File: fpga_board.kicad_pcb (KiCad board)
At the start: 8 copper layers, 50 x 50 mm, 157 parts, among them Q1 2N7002PW, Q2 2N7002PW, Q3 2N7002PW, Q4 2N7002PW, Q5 2N7002PW, Q6 2N7002PW, SW1 1TS028A-1300-0600-CT, U1 LFE5U-45F-7BG256I, U10 TLV62569DRL, U2 CYUSB3014-BZXC, U3 TLV62569DRL, U5 K4B4G1646E-BCMA, U6 K4B4G1646E-BCMA, U7 TLV62569DRL, U8 TLV62569DRL, U9 TLV62569DRL, X1 XO32, Y1 Crystal_GND24

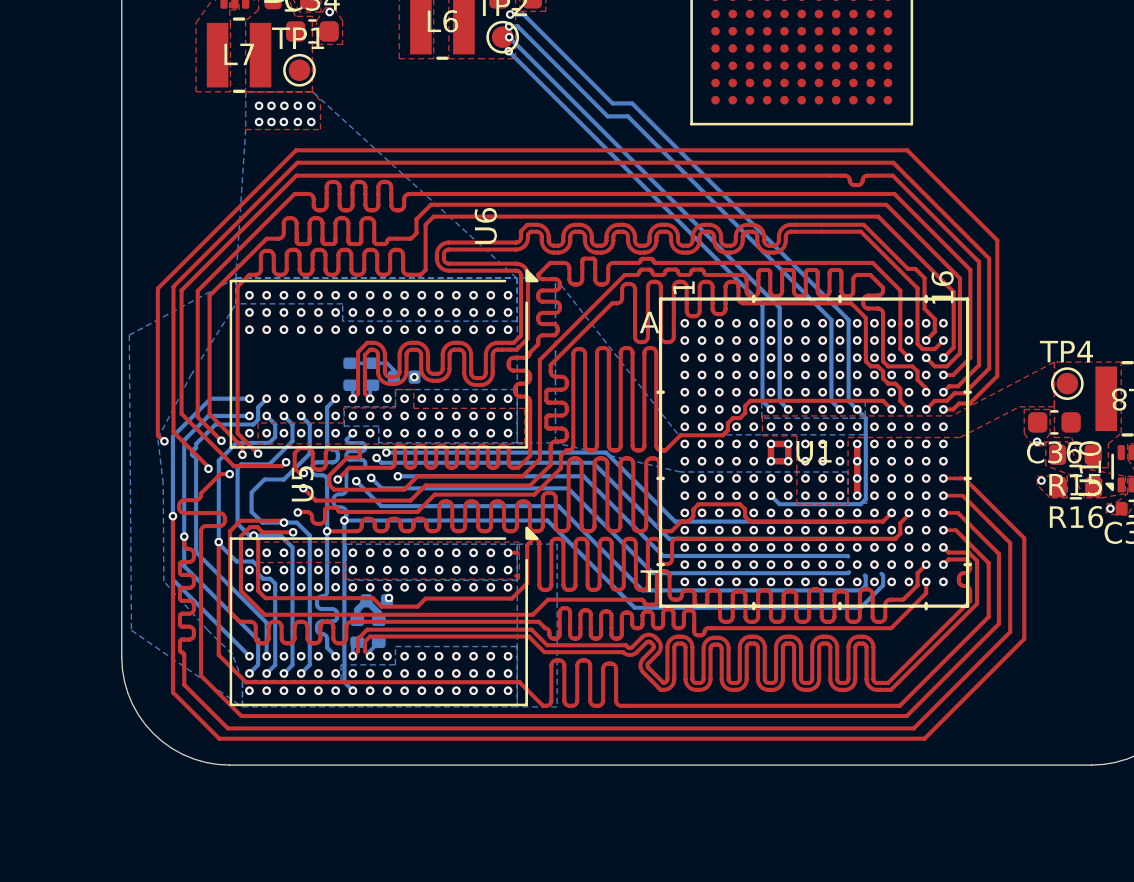
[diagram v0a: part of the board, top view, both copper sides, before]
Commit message: ACC pins completed.
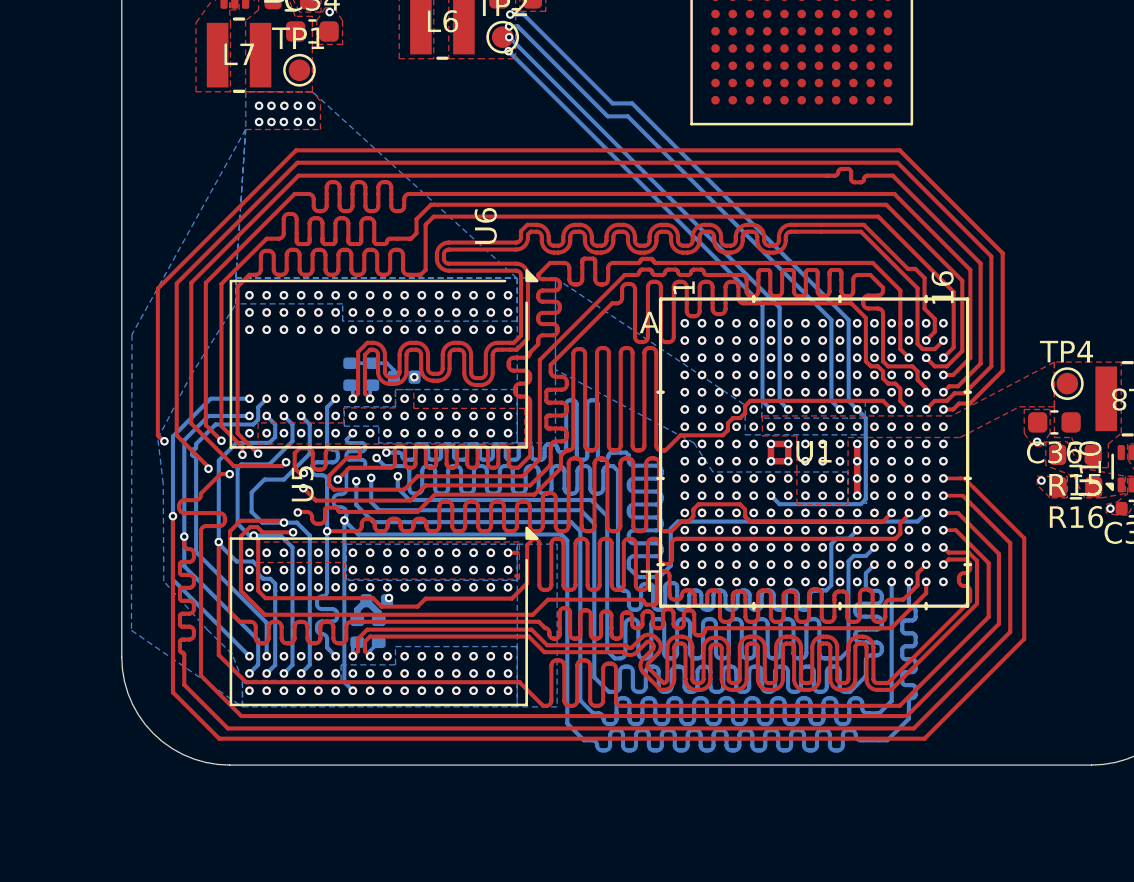
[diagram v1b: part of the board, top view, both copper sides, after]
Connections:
- U1 pad M15: unconnected-(U1B-PR35D-PadM15) -> ACC.#RAS
- U1 pad N11: unconnected-(U1B-PR68B-PadN11) -> ACC.ODT
- U1 pad P12: unconnected-(U1B-PR68D-PadP12) -> ACC.#CAS
- U1 pad R12: unconnected-(U1B-PR65A-PadR12) -> ACC.#WE
- U1 pad T13: unconnected-(U1B-PR65B-PadT13) -> ACC.BA2
- U1 pad T14: unconnected-(U1B-PR62D-PadT14) -> ACC.CKE
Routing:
- net ACC.#CAS: track 38.4 -> 75.6 mm, vias 3 -> 4
- net ACC.#RAS: track 38.6 -> 75.6 mm, vias 3 -> 4
- net ACC.ODT: track 39.4 -> 75.3 mm, vias 3 -> 4
- net ACC.#WE: track 40.0 -> 75.5 mm, vias 3 -> 4
- net ACC.BA2: track 42.0 -> 75.3 mm, vias 3 -> 4
- net ACC.CKE: track 43.6 -> 75.5 mm, vias 3 -> 4
- net unconnected-(U1B-PR68D-PadP12): vias 1 -> 0
- net unconnected-(U1B-PR68B-PadN11): vias 1 -> 0
- net unconnected-(U1B-PR65B-PadT13): vias 1 -> 0
- net unconnected-(U1B-PR65A-PadR12): vias 1 -> 0
- net unconnected-(U1B-PR62D-PadT14): vias 1 -> 0
- net unconnected-(U1B-PR35D-PadM15): vias 1 -> 0
- added copper zone on In6.Cu, net GND
